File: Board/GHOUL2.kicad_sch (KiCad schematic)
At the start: 36 parts, among them M1 Motor_Servo, U1 Teensy4.1, U2 DS18S20, U4 TPS62133, U5 MS5607-02BA, U6 SAM-M8Q

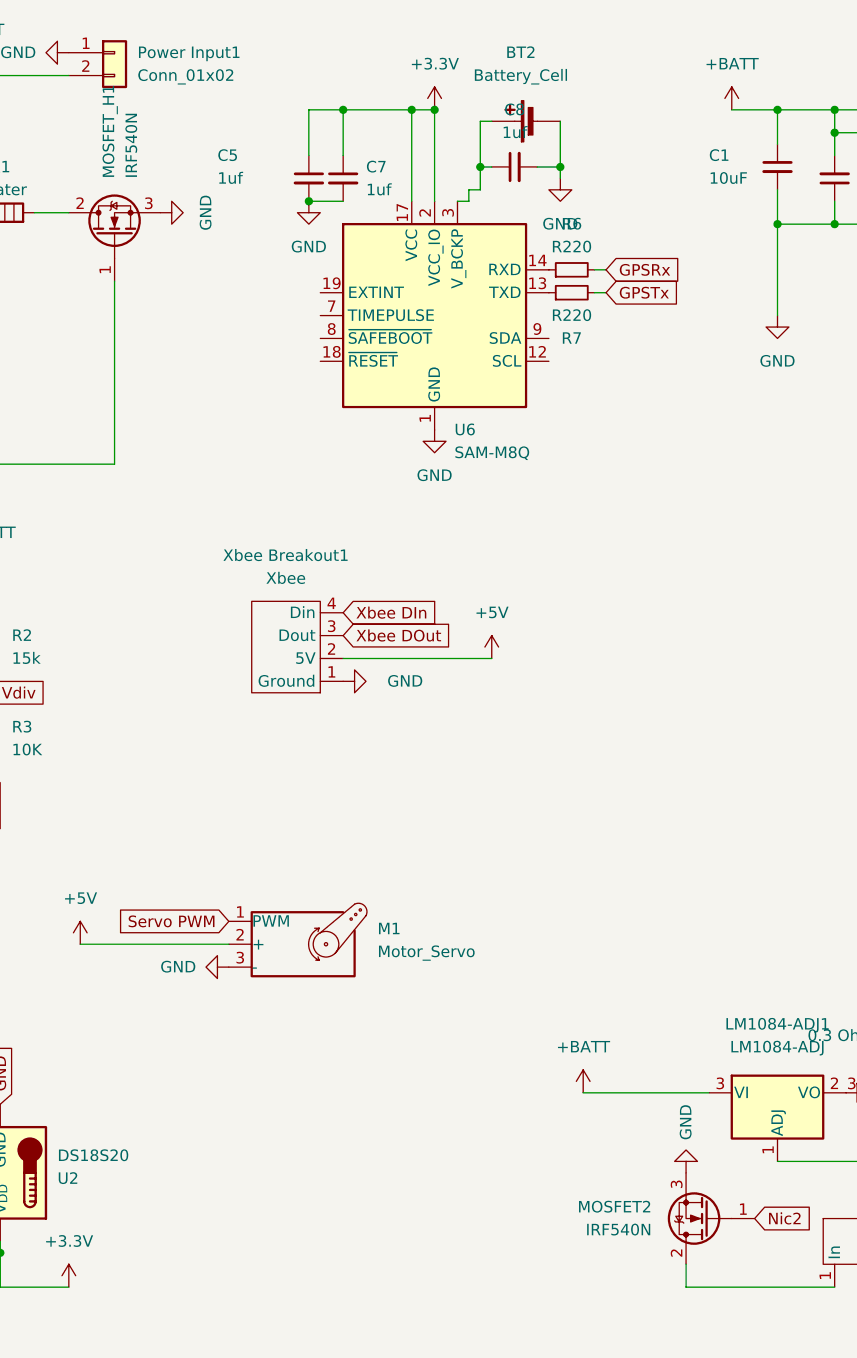
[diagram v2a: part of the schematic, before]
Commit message: fixed more things
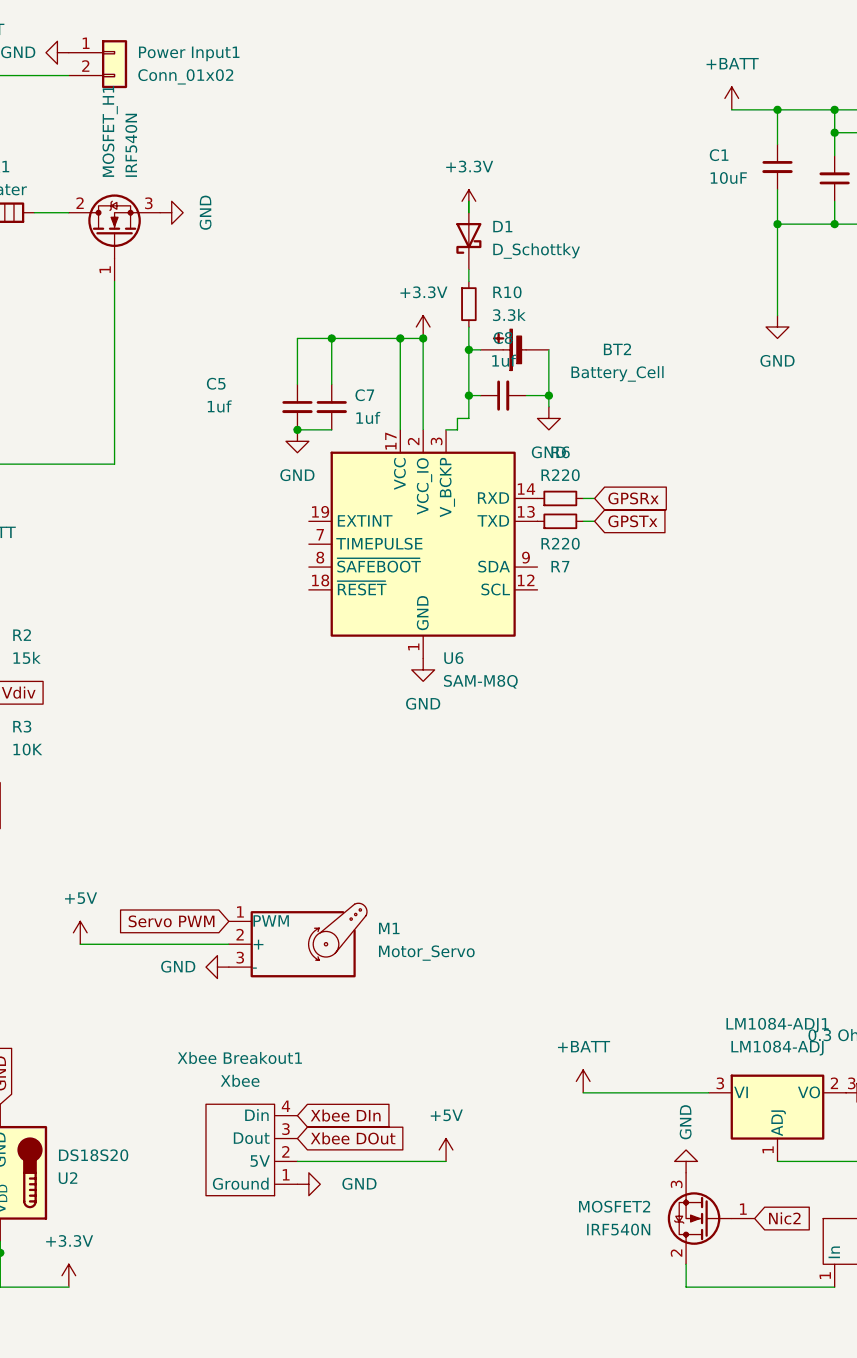
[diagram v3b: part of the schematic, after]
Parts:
- added D1: D_Schottky, Diode_SMD:D_SOD-123F, symbol Device:D_Schottky
- added R10: 3.3k, Resistor_SMD:R_0201_0603Metric_Pad0.64x0.40mm_HandSolder, symbol Device:R_Small
- BT2: footprint Battery:BatteryHolder_Keystone_2998_1x6.8mm -> ML414H_IV01E:SEIKO_ML414H_IV01E
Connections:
- net +3.3V: now also D1.2 (A)
- net at BT2.1 (+), C8.1, U6.3 (V_BCKP): now also R10.2
- new net: D1.1 (K), R10.1
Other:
- moved on the sheet: BT2, C5, C7, C8, R6, R7, U6, Xbee Breakout1
